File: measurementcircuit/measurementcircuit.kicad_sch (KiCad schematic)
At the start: 81 parts, among them J1 Conn_01x02, J10 Conn_01x02, J11 Conn_01x02, J12 Conn_01x02, J13 250-108/000-006, J15 Conn_01x02, J16 Conn_01x02, J17 250-116/000-012, J18 2604-3102, J19 2604-3102, J2 Conn_01x02, J20 2604-3102, J21 Conn_01x02, J22 Conn_01x02, J23 Conn_01x02, J24 Conn_01x02, J25 Conn_01x02, J26 Conn_01x02, J27 Conn_01x02, J28 Conn_01x02, J29 Conn_01x02, J3 2604-3102, J30 Conn_01x02, J31 Conn_01x02, J32 Conn_01x02, J33 Conn_01x02, J34 Conn_01x02, J35 Conn_01x02, J36 Conn_01x02, J37 Conn_01x02, J38 Conn_01x02, J39 Conn_01x02, J4 2604-3102, J40 Conn_01x02, J41 Conn_01x02, J42 Conn_01x02, J5 2604-3102, J6 2604-3102, J7 2604-3102, J8 Conn_01x02, J9 Conn_01x02

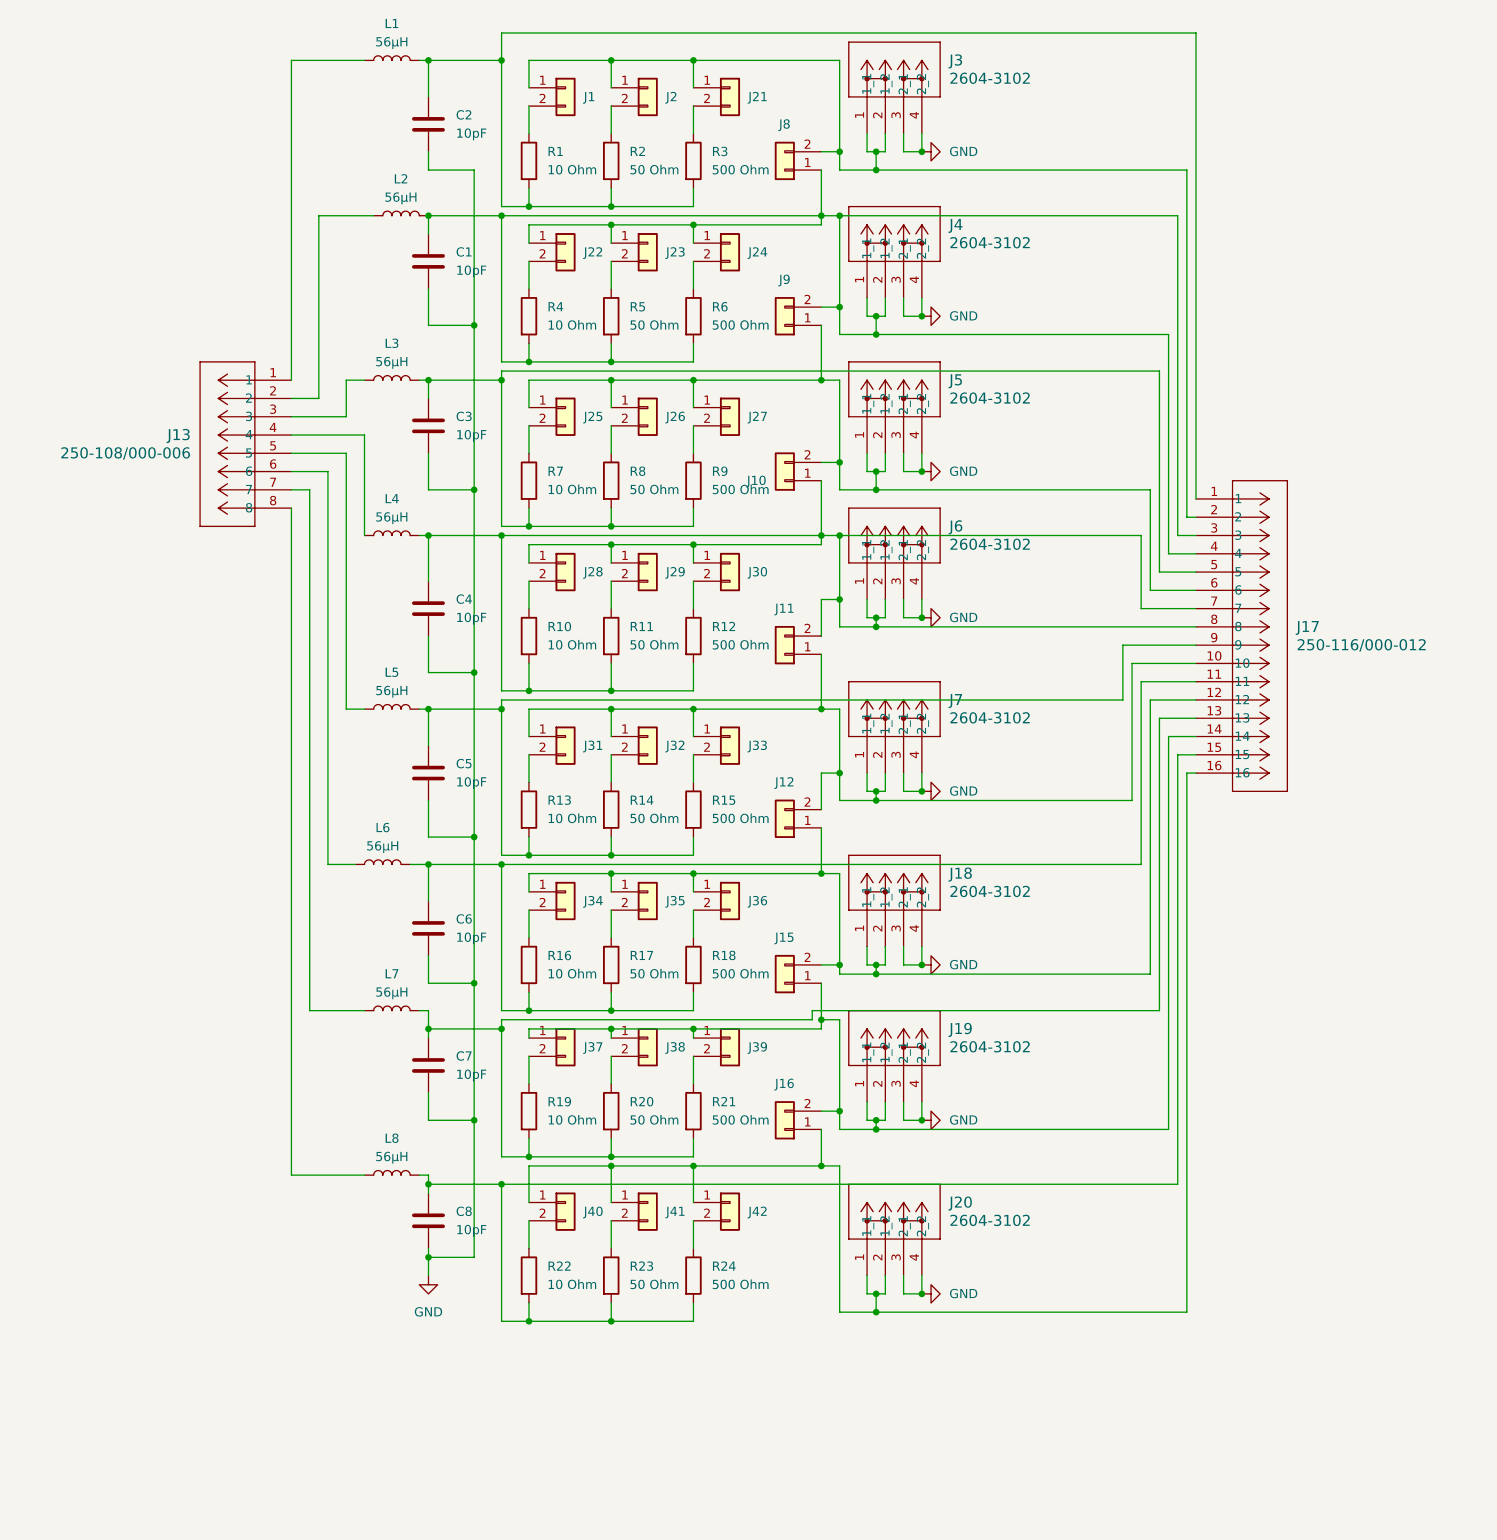
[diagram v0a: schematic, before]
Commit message: Resize canvas
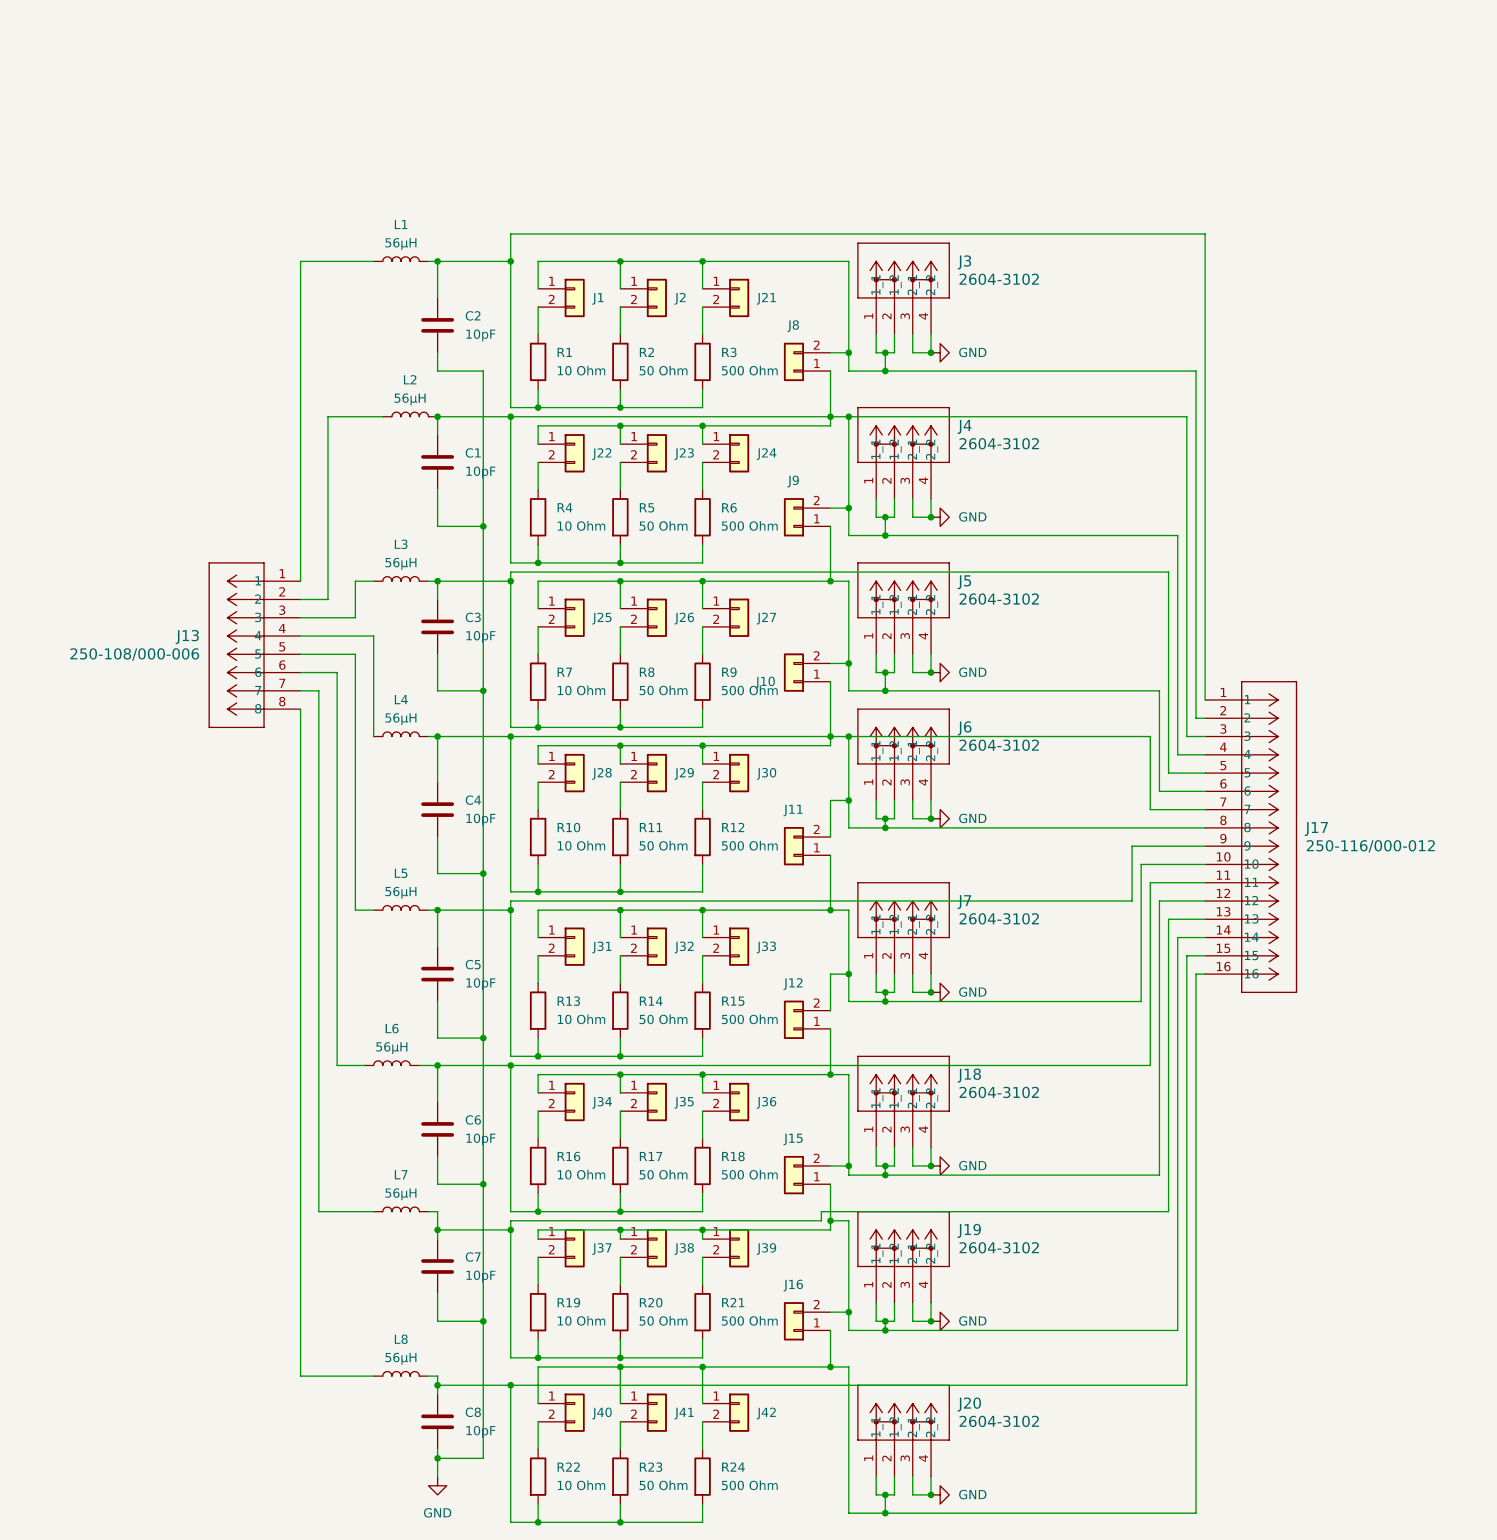
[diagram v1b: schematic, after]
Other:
- title: (none) -> Measurement Circuit
- moved on the sheet: C1, C2, C3, C4, C5, C6, C7, C8, J1, J10, J11, J12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
